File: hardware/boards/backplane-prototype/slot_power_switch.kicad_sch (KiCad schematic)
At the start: 14 parts, among them Q1 SQD50P06-15L_GE3, Q2 BSS123, U1 74HC595D,118

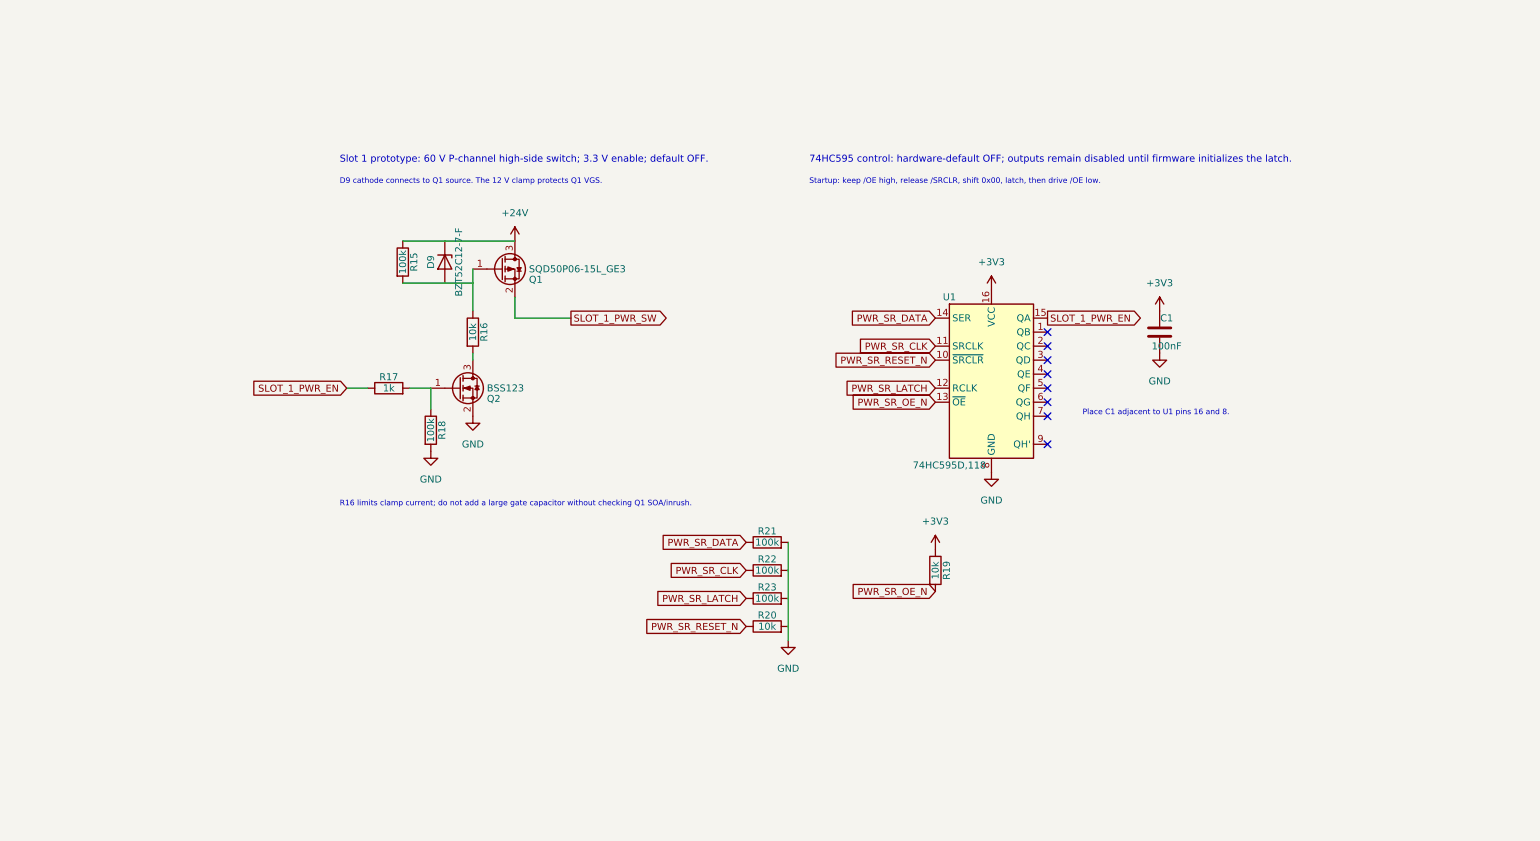
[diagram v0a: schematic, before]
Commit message: chore: checkpoint current board layout
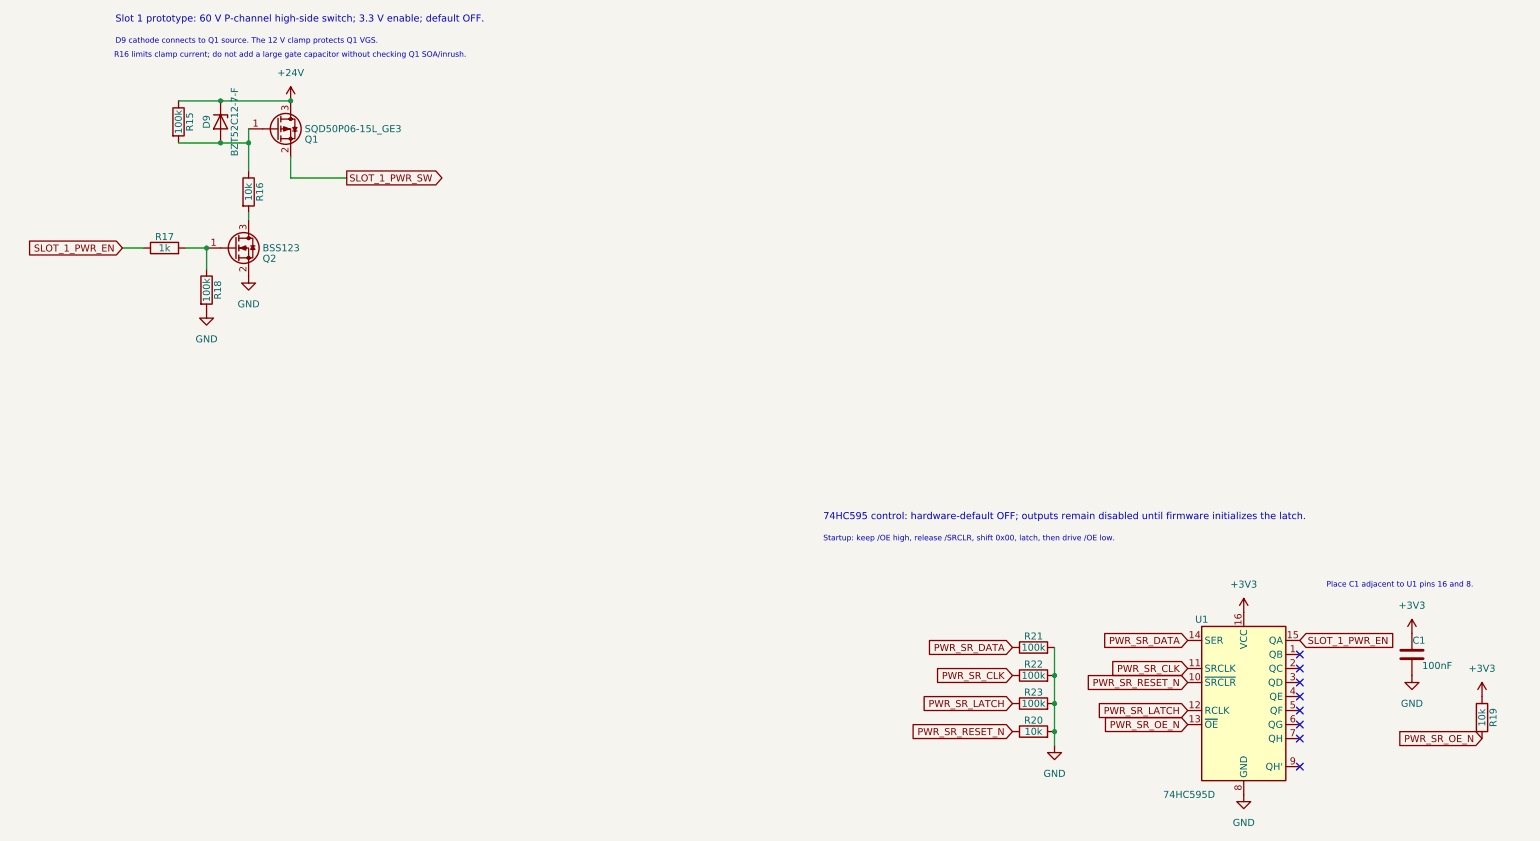
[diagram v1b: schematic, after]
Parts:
- U1: value 74HC595D,118 -> 74HC595D
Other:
- title: Slot 1 High-Side Power Switch -> Backplane Prototype
- moved on the sheet: C1, D9, Q1, Q2, R15, R16, R17, R18, R19, R20, R21, R22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
